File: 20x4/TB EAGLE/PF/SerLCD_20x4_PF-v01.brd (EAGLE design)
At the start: 73.7 x 99.1 mm, 5 parts

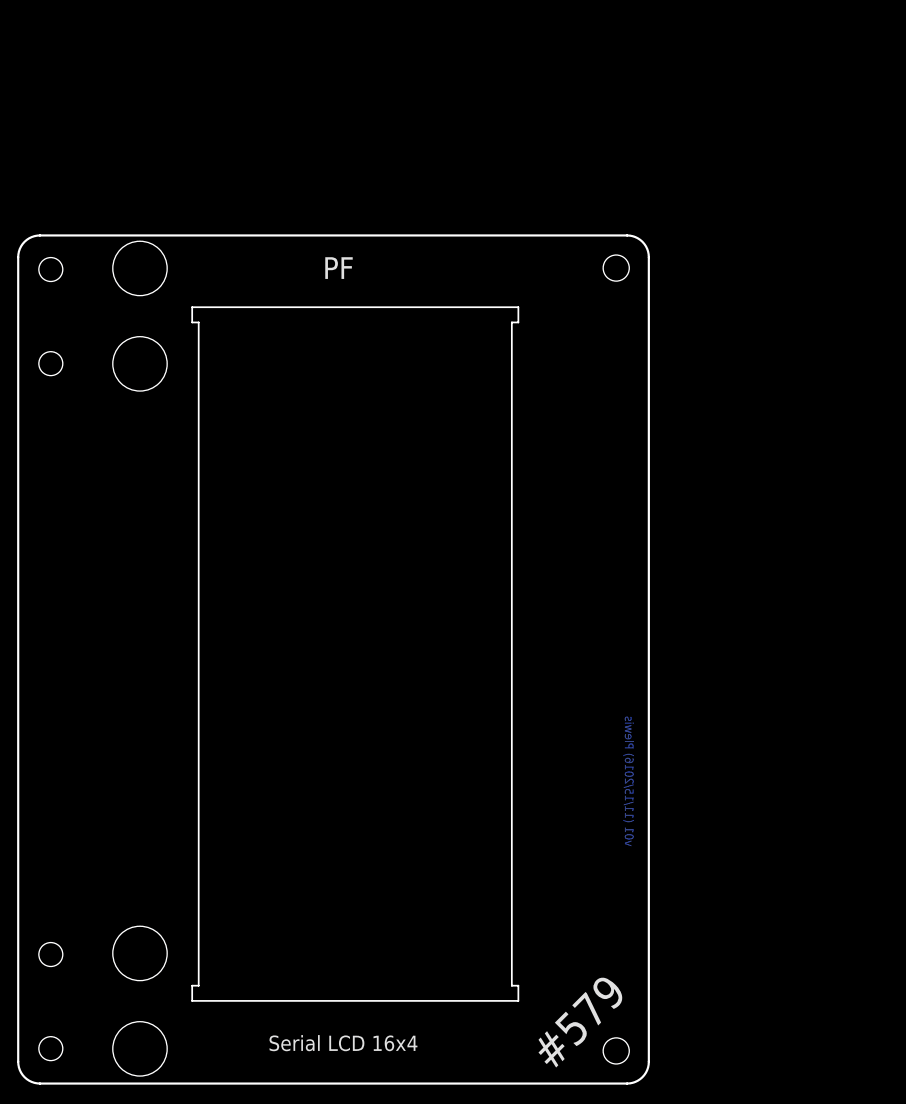
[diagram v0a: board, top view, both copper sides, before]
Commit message: finshed up 20x4, RFR
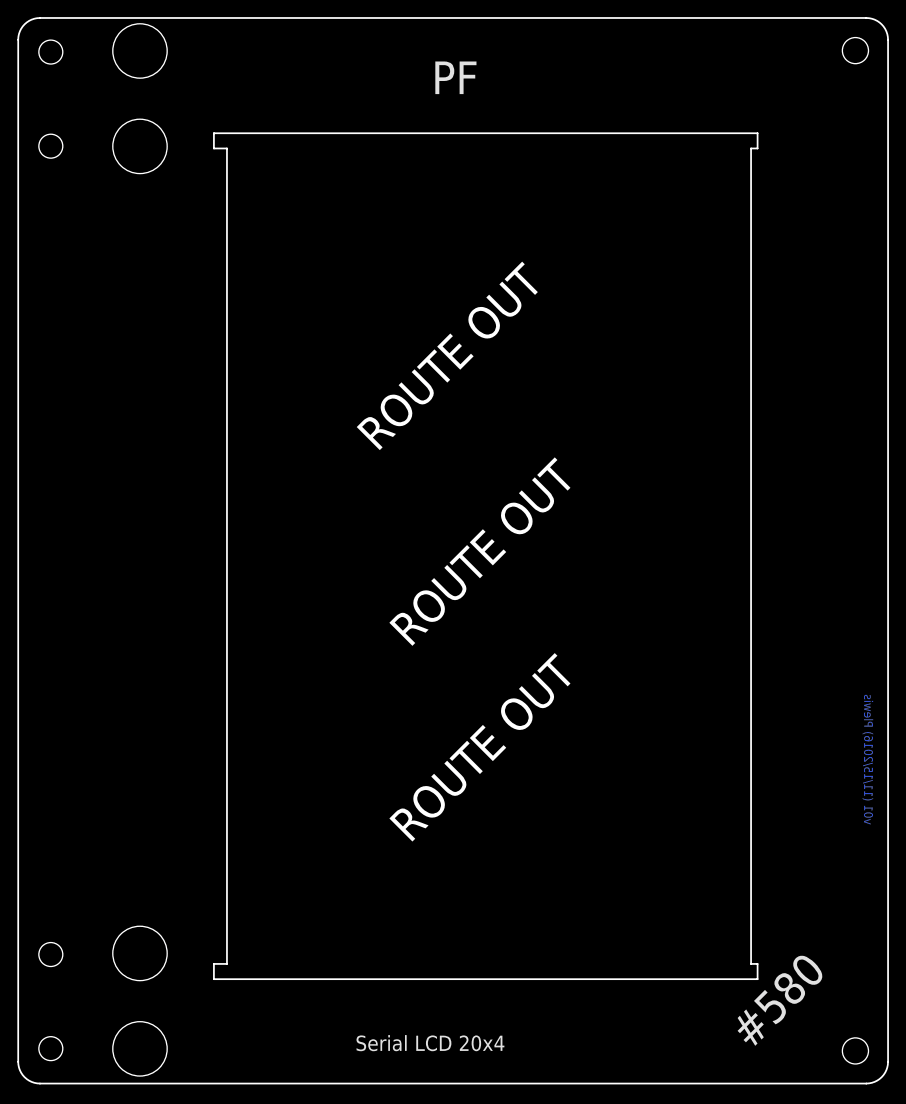
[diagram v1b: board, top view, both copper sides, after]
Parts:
- removed U$2: (no value), SerLCD_dimensions:SRE_LCD_16X2_REF_ONLY
- added U$1: (no value), SerLCD_dimensions:SER_LCD_20X4_REF_ONLY
- moved U$3 37.8 mm to (97.8, 120.7)
- moved U$8 27.9 mm to (97.8, 3.81)
- moved U$6 25.4 mm to (0.00, 105.4)
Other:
- board size 73.7 x 99.1 mm -> 101.6 x 124.5 mm
- board text added: "#580"
- board text added: "ROUTE OUT"
- board text added: "Serial LCD 20x4"
- board text removed: "#579"
- board text removed: "Serial LCD 16x4"
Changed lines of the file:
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@@
 <grid distance="0.05" unitdist="inch" unit="inch" style="lines" multiple="1" display="yes" altdistance="0.005" altunitdist="inch" altunit="inch"/>
 <layers>
-<layer number="1" name="Top" color="4" fill="1" visible="no" active="yes"/>
+<layer number="1" name="Top" color="4" fill="1" visible="yes" active="yes"/>
 <layer number="2" name="Route2" color="1" fill="3" visible="no" active="no"/>
 <layer number="3" name="Route3" color="4" fill="3" visible="no" active="no"/>
@@
 <layer number="14" name="Route14" color="1" fill="6" visible="no" active="no"/>
 <layer number="15" name="Route15" color="4" fill="6" visible="no" active="no"/>
-<layer number="16" name="Bottom" color="1" fill="1" visible="no" active="yes"/>
-<layer number="17" name="Pads" color="2" fill="1" visible="no" active="yes"/>
-<layer number="18" name="Vias" color="2" fill="1" visible="no" active="yes"/>
-<layer number="19" name="Unrouted" color="6" fill="1" visible="no" active="yes"/>
+<layer number="16" name="Bottom" color="1" fill="1" visible="yes" active="yes"/>
+<layer number="17" name="Pads" color="2" fill="1" visible="yes" active="yes"/>
+<layer number="18" name="Vias" color="2" fill="1" visible="yes" active="yes"/>
+<layer number="19" name="Unrouted" color="6" fill="1" visible="yes" active="yes"/>
 <layer number="20" name="Dimension" color="15" fill="1" visible="yes" active="yes"/>
 <layer number="21" name="tPlace" color="16" fill="1" visible="yes" active="yes"/>
-<layer number="22" name="bPlace" color="14" fill="1" visible="no" active="yes"/>
-<layer number="23" name="tOrigins" color="15" fill="1" visible="no" active="yes"/>
-<layer number="24" name="bOrigins" color="15" fill="1" visible="no" active="yes"/>
+<layer number="22" name="bPlace" color="14" fill="1" visible="yes" active="yes"/>
+<layer number="23" name="tOrigins" color="15" fill="1" visible="yes" active="yes"/>
+<layer number="24" name="bOrigins" color="15" fill="1" visible="yes" active="yes"/>
 <layer number="25" name="tNames" color="7" fill="1" visible="no" active="yes"/>
 <layer number="26" name="bNames" color="7" fill="1" visible="no" active="yes"/>
@@
 <layer number="43" name="vRestrict" color="2" fill="10" visible="no" active="yes"/>
 <layer number="44" name="Drills" color="7" fill="1" visible="no" active="yes"/>
-<layer number="45" name="Holes" color="7" fill="1" visible="no" active="yes"/>
+<layer number="45" name="Holes" color="7" fill="1" visible="yes" active="yes"/>
 <layer number="46" name="Milling" color="3" fill="1" visible="no" active="yes"/>
 <layer number="47" name="Measures" color="7" fill="1" visible="no" active="yes"/>
 <layer number="48" name="Document" color="7" fill="1" visible="no" active="yes"/>
-<layer number="49" name="Reference" color="13" fill="1" visible="no" active="yes"/>
+<layer number="49" name="Reference" color="13" fill="1" visible="yes" active="yes"/>
 <layer number="50" name="dxf" color="7" fill="1" visible="no" active="yes"/>
-<layer number="51" name="tDocu" color="6" fill="1" visible="no" active="yes"/>
+<layer number="51" name="tDocu" color="6" fill="1" visible="yes" active="yes"/>
 <layer number="52" name="bDocu" color="7" fill="1" visible="no" active="yes"/>
 <layer number="53" name="tGND_GNDA" color="7" fill="9" visible="no" active="no"/>
@@
 <board>
 <plain>
-<wire x1="2.54" y1="0" x2="0" y2="2.54" width="0.254" layer="20" curve="-90"/>
-<wire x1="0" y1="2.54" x2="0" y2="96.52" width="0.254" layer="20"/>
-<wire x1="0" y1="96.52" x2="2.54" y2="99.06" width="0.254" layer="20" curve="-90"/>
-<wire x1="2.54" y1="99.06" x2="71.12" y2="99.06" width="0.254" layer="20"/>
-<wire x1="71.12" y1="99.06" x2="73.66" y2="96.52" width="0.254" layer="20" curve="-90"/>
-<wire x1="73.66" y1="96.52" x2="73.66" y2="2.54" width="0.254" layer="20"/>
-<wire x1="73.66" y1="2.54" x2="71.12" y2="0" width="0.254" layer="20" curve="-90"/>
-<wire x1="71.12" y1="0" x2="2.54" y2="0" width="0.254" layer="20"/>
-<wire x1="73.66" y1="96.52" x2="71.12" y2="99.06" width="0.254" layer="49" curve="90"/>
-<wire x1="71.12" y1="99.06" x2="1.27" y2="99.06" width="0.254" layer="49"/>
-<wire x1="1.27" y1="99.06" x2="0" y2="96.52" width="0.254" layer="49" curve="90"/>
-<text x="29.21" y="3.81" size="1.778" layer="21" ratio="15">Serial LCD 16x4</text>
-<text x="71.882" y="42.926" size="1.016" layer="16" font="vector" ratio="15" rot="MR270">v01 (11/15/2016) Plewis</text>
-<text x="62.23" y="1.27" size="3.81" layer="21" font="vector" ratio="15" rot="R45">#579</text>
-<wire x1="0" y1="96.52" x2="0" y2="2.54" width="0.254" layer="49"/>
-<wire x1="0" y1="2.54" x2="2.54" y2="0" width="0.254" layer="49" curve="90"/>
-<wire x1="2.54" y1="0" x2="71.12" y2="0" width="0.254" layer="49"/>
-<wire x1="71.12" y1="0" x2="73.66" y2="2.54" width="0.254" layer="49" curve="90"/>
-<wire x1="20.32" y1="90.678" x2="20.32" y2="88.9" width="0.2032" layer="20"/>
-<wire x1="20.32" y1="88.9" x2="21.082" y2="88.9" width="0.2032" layer="20"/>
-<wire x1="21.082" y1="88.9" x2="21.082" y2="11.43" width="0.2032" layer="20"/>
-<wire x1="21.082" y1="11.43" x2="20.32" y2="11.43" width="0.2032" layer="20"/>
-<wire x1="20.32" y1="11.43" x2="20.32" y2="9.652" width="0.2032" layer="20"/>
-<wire x1="20.32" y1="9.652" x2="58.42" y2="9.652" width="0.2032" layer="20"/>
-<wire x1="58.42" y1="9.652" x2="58.42" y2="11.43" width="0.2032" layer="20"/>
-<wire x1="58.42" y1="11.43" x2="57.658" y2="11.43" width="0.2032" layer="20"/>
-<wire x1="57.658" y1="11.43" x2="57.658" y2="88.9" width="0.2032" layer="20"/>
-<wire x1="57.658" y1="88.9" x2="58.42" y2="88.9" width="0.2032" layer="20"/>
-<wire x1="58.42" y1="88.9" x2="58.42" y2="90.678" width="0.2032" layer="20"/>
-<wire x1="58.42" y1="90.678" x2="20.32" y2="90.678" width="0.2032" layer="20"/>
-<text x="35.56" y="93.98" size="2.54" layer="21" font="vector" ratio="15">PF</text>
+<wire x1="2.54" y1="0" x2="0" y2="2.54" width="0.2032" layer="20" curve="-90"/>
+<wire x1="0" y1="2.54" x2="0" y2="121.92" width="0.2032" layer="20"/>
+<wire x1="0" y1="121.92" x2="2.54" y2="124.46" width="0.2032" layer="20" curve="-90"/>
+<wire x1="2.54" y1="124.46" x2="99.06" y2="124.46" width="0.2032" layer="20"/>
+<wire x1="99.06" y1="124.46" x2="101.6" y2="121.92" width="0.2032" layer="20" curve="-90"/>
+<wire x1="101.6" y1="121.92" x2="101.6" y2="2.54" width="0.2032" layer="20"/>
+<wire x1="101.6" y1="2.54" x2="99.06" y2="0" width="0.2032" layer="20" curve="-90"/>
+<wire x1="99.06" y1="0" x2="2.54" y2="0" width="0.2032" layer="20"/>
+<wire x1="101.6" y1="121.92" x2="99.06" y2="124.46" width="0.2032" layer="49" curve="90"/>
+<wire x1="99.06" y1="124.46" x2="1.27" y2="124.46" width="0.2032" layer="49"/>
+<wire x1="1.27" y1="124.46" x2="0" y2="121.92" width="0.2032" layer="49" curve="90"/>
+<text x="39.37" y="3.81" size="1.778" layer="21" ratio="15">Serial LCD 20x4</text>
+<text x="99.822" y="45.466" size="1.016" layer="16" font="vector" ratio="15" rot="MR270">v01 (11/15/2016) Plewis</text>
+<text x="85.48905" y="3.81" size="3.81" layer="21" font="vector" ratio="15" rot="R45">#580</text>
+<wire x1="0" y1="121.92" x2="0" y2="2.54" width="0.2032" layer="49"/>
+<wire x1="0" y1="2.54" x2="2.54" y2="0" width="0.2032" layer="49" curve="90"/>
+<wire x1="2.54" y1="0" x2="99.06" y2="0" width="0.2032" layer="49"/>
+<wire x1="99.06" y1="0" x2="101.6" y2="2.54" width="0.2032" layer="49" curve="90"/>
+<text x="48.26" y="115.57" size="3.81" layer="21" font="vector" ratio="15">PF</text>
+<wire x1="86.36" y1="110.998" x2="22.86" y2="110.998" width="0.2032" layer="20"/>
+<wire x1="22.86" y1="110.998" x2="22.86" y2="109.22" width="0.2032" layer="20"/>
+<wire x1="22.86" y1="109.22" x2="24.384" y2="109.22" width="0.2032" layer="20"/>
+<wire x1="24.384" y1="109.22" x2="24.384" y2="13.97" width="0.2032" layer="20"/>
+<wire x1="24.384" y1="13.97" x2="22.86" y2="13.97" width="0.2032" layer="20"/>
+<wire x1="22.86" y1="13.97" x2="22.86" y2="12.192" width="0.2032" layer="20"/>
+<wire x1="22.86" y1="12.192" x2="86.36" y2="12.192" width="0.2032" layer="20"/>
+<wire x1="86.36" y1="12.192" x2="86.36" y2="13.97" width="0.2032" layer="20"/>
+<wire x1="86.36" y1="13.97" x2="85.598" y2="13.97" width="0.2032" layer="20"/>
+<wire x1="85.598" y1="13.97" x2="85.598" y2="109.22" width="0.2032" layer="20"/>
+<wire x1="85.598" y1="109.22" x2="86.36" y2="109.22" width="0.2032" layer="20"/>
+<wire x1="86.36" y1="109.22" x2="86.36" y2="110.998" width="0.2032" layer="20"/>
+<text x="41.91" y="73.66" size="3.81" layer="20" font="vector" ratio="15" rot="R45">ROUTE OUT</text>
+<text x="45.72" y="50.8" size="3.81" layer="20" font="vector" ratio="15" rot="R45">ROUTE OUT</text>
+<text x="45.72" y="27.94" size="3.81" layer="20" font="vector" ratio="15" rot="R45">ROUTE OUT</text>
 </plain>
 <attributes>
@@
 </autorouter>
 <elements>
-<element name="U$3" library="SparkFun" package="STAND-OFF-TIGHT" value="" x="69.85" y="95.25"/>
-<element name="U$8" library="SparkFun" package="STAND-OFF-TIGHT" value="" x="69.85" y="3.81"/>
-<element name="U$6" library="Testing" package="GOLD_HINGE_PM" value="GOLD_HINDGEPM+PF" x="0" y="80.01"/>
+<element name="U$3" library="SparkFun" package="STAND-OFF-TIGHT" value="" x="97.79" y="120.65"/>
+<element name="U$8" library="SparkFun" package="STAND-OFF-TIGHT" value="" x="97.79" y="3.81"/>
+<element name="U$6" library="Testing" package="GOLD_HINGE_PM" value="GOLD_HINDGEPM+PF" x="0" y="105.41"/>
 <element name="U$7" library="Testing" package="GOLD_HINGE_PM" value="GOLD_HINDGEPM+PF" x="0" y="0"/>
-<element name="U$2" library="SerLCD_dimensions" package="SRE_LCD_16X2_REF_ONLY" value="" x="57.15" y="10.16" rot="R90"/>
+<element name="U$1" library="SerLCD_dimensions" package="SER_LCD_20X4_REF_ONLY" value="" x="85.09" y="12.7" rot="R90"/>
 </elements>
 <signals>
